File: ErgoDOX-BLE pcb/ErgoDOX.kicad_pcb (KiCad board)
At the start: 2 copper layers, 182.8 x 158.9 mm, 110 parts, among them J1 Conn_01x04, J2 Conn_01x02_Female, J3 Conn_01x02_Female, J4 Conn_01x02, J5 Conn_01x02, P1 USB_C_Plug_USB2.0, Q1 Q_NPN_BCE, SW0:10 SW0:3, SW0:11 SW0:2, SW0:12 SW0:1, SW0:7 SW0:6, SW0:8 SW0:5, SW0:9 SW0:4, SW1:10 SW1:3, SW1:11 SW1:2, SW1:12 SW1:1, SW1:13 SW1:0, SW1:9 SW1:4, SW2:10 SW2:3, SW2:11 SW2:2, SW2:12 SW2:1, SW2:13 SW2:0, SW2:7 SW2:6, SW2:8 SW2:5, SW2:9 SW2:4, SW3:10 SW3:3, SW3:11 SW3:2, SW3:12 SW3:1, SW3:13 SW3:0, SW3:8 SW3:5, SW3:9 SW3:4, SW4:10 SW4:3, SW4:11 SW4:2, SW4:12 SW4:1, SW4:13 SW4:0, SW4:7 SW4:6, SW4:8 SW4:5, SW4:9 SW4:4, SW5:10 SW5:3, SW5:11 SW5:2, SW5:12 SW5:1, SW5:13 SW5:0, SW5:7 SW5:6, SW5:8 SW5:5, SW5:9 SW5:4, U1 MCP23018, U3 C0720B001F

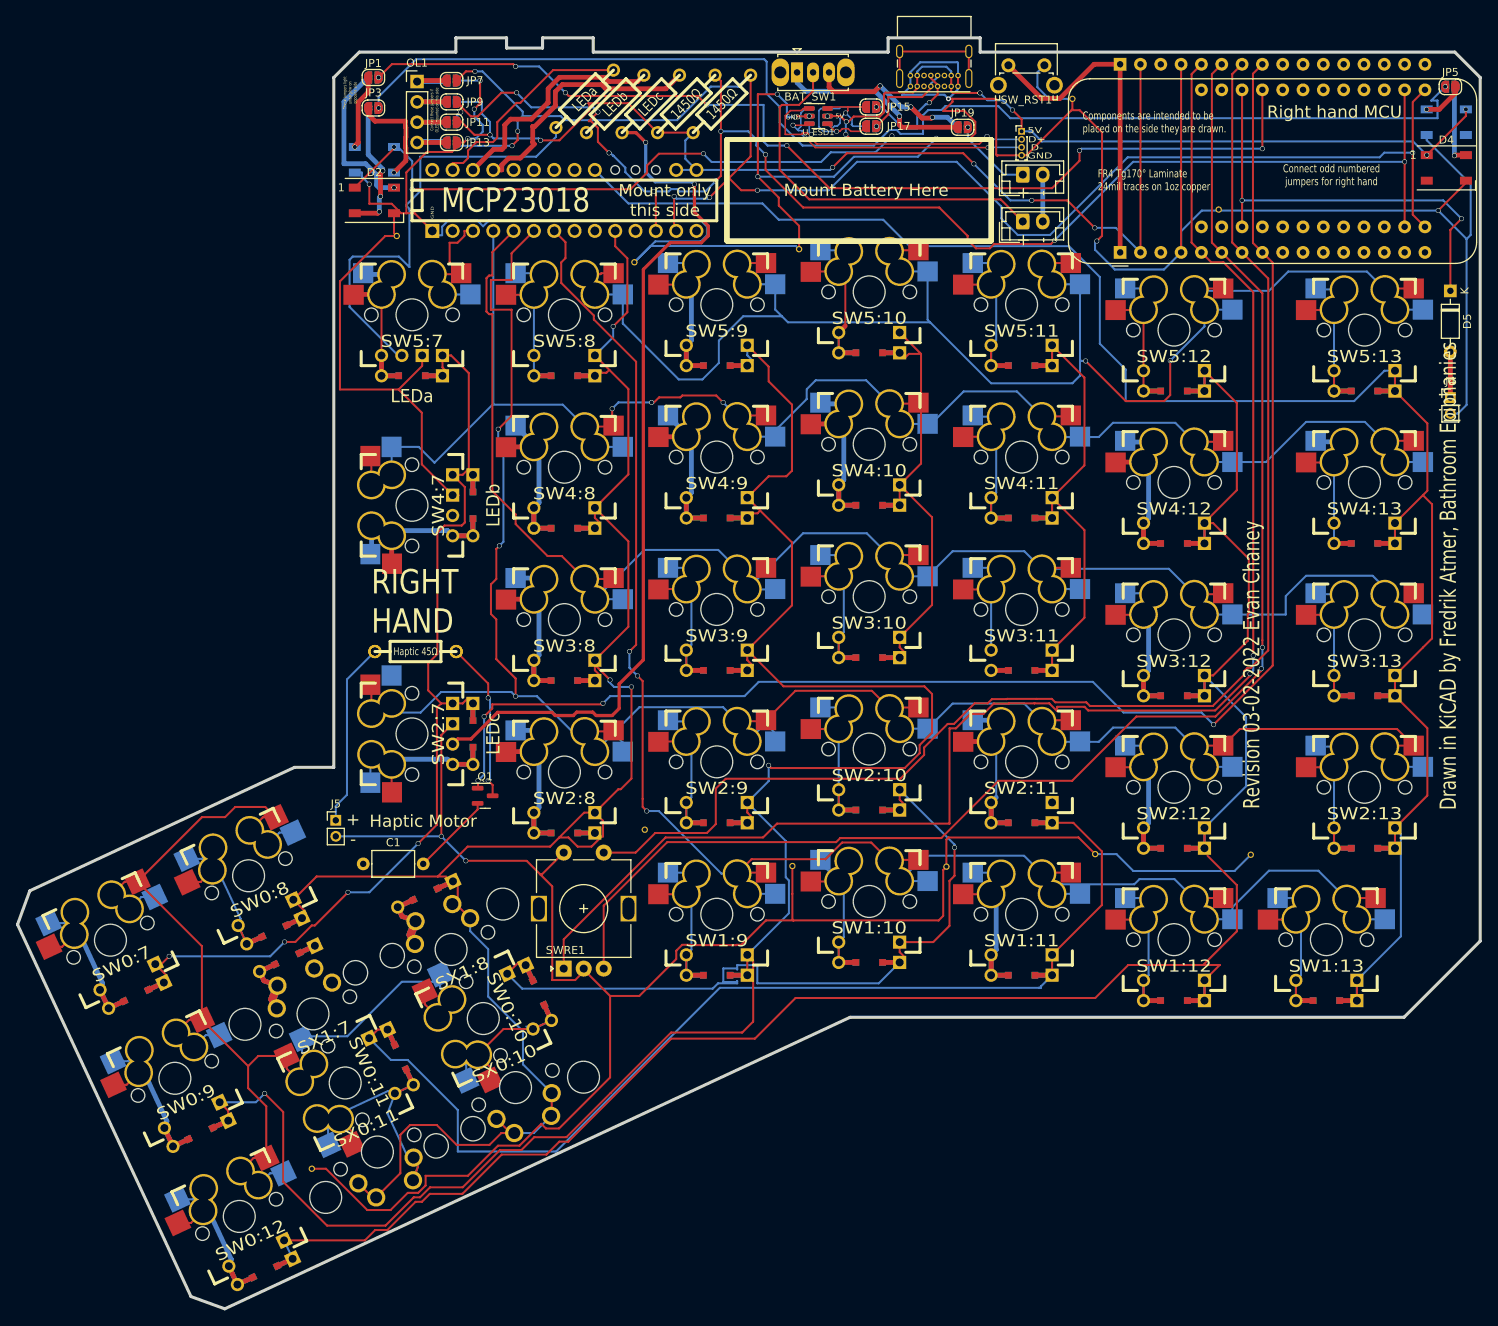
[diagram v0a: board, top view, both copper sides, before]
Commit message: Route me daddy
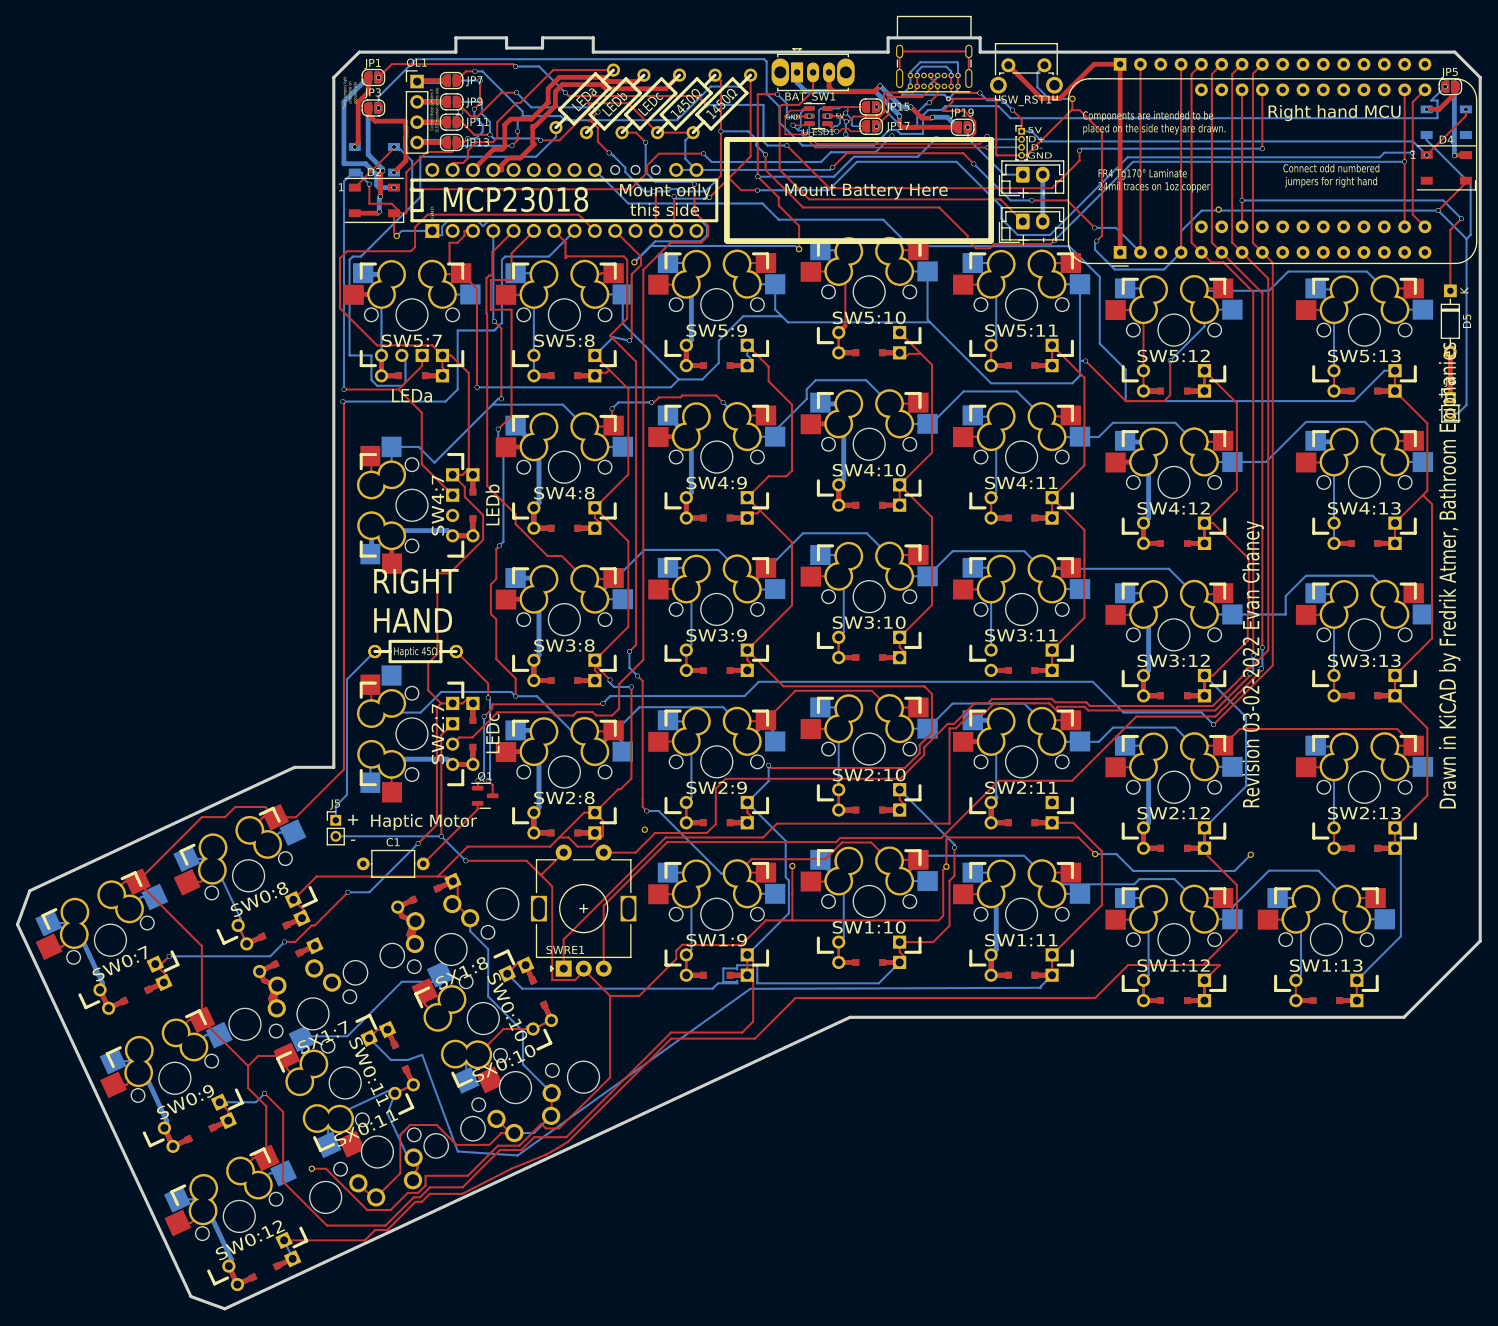
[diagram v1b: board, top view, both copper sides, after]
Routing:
- net /ROW0: track 139.8 -> 243.9 mm, vias 0 -> 1
- net /COL6: track 116.4 -> 175.9 mm
- net /COL3: track 92.1 -> 143.1 mm
- net /ROW4: track 255.8 -> 206.9 mm, vias 3 -> 5
- net /ROW5: track 222.4 -> 263.1 mm, vias 2 -> 3
- net /ROW1: track 218.1 -> 224.0 mm
- net Net-(LED_A1-Pad1): track 57.0 -> 62.4 mm
- net GND: track 661.7 -> 666.6 mm, vias 14 -> 15
- net /COL5: track 218.9 -> 222.0 mm
- net /COL1: track 250.7 -> 249.6 mm
- net /COL2: track 179.1 -> 178.0 mm

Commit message: Everything is connected
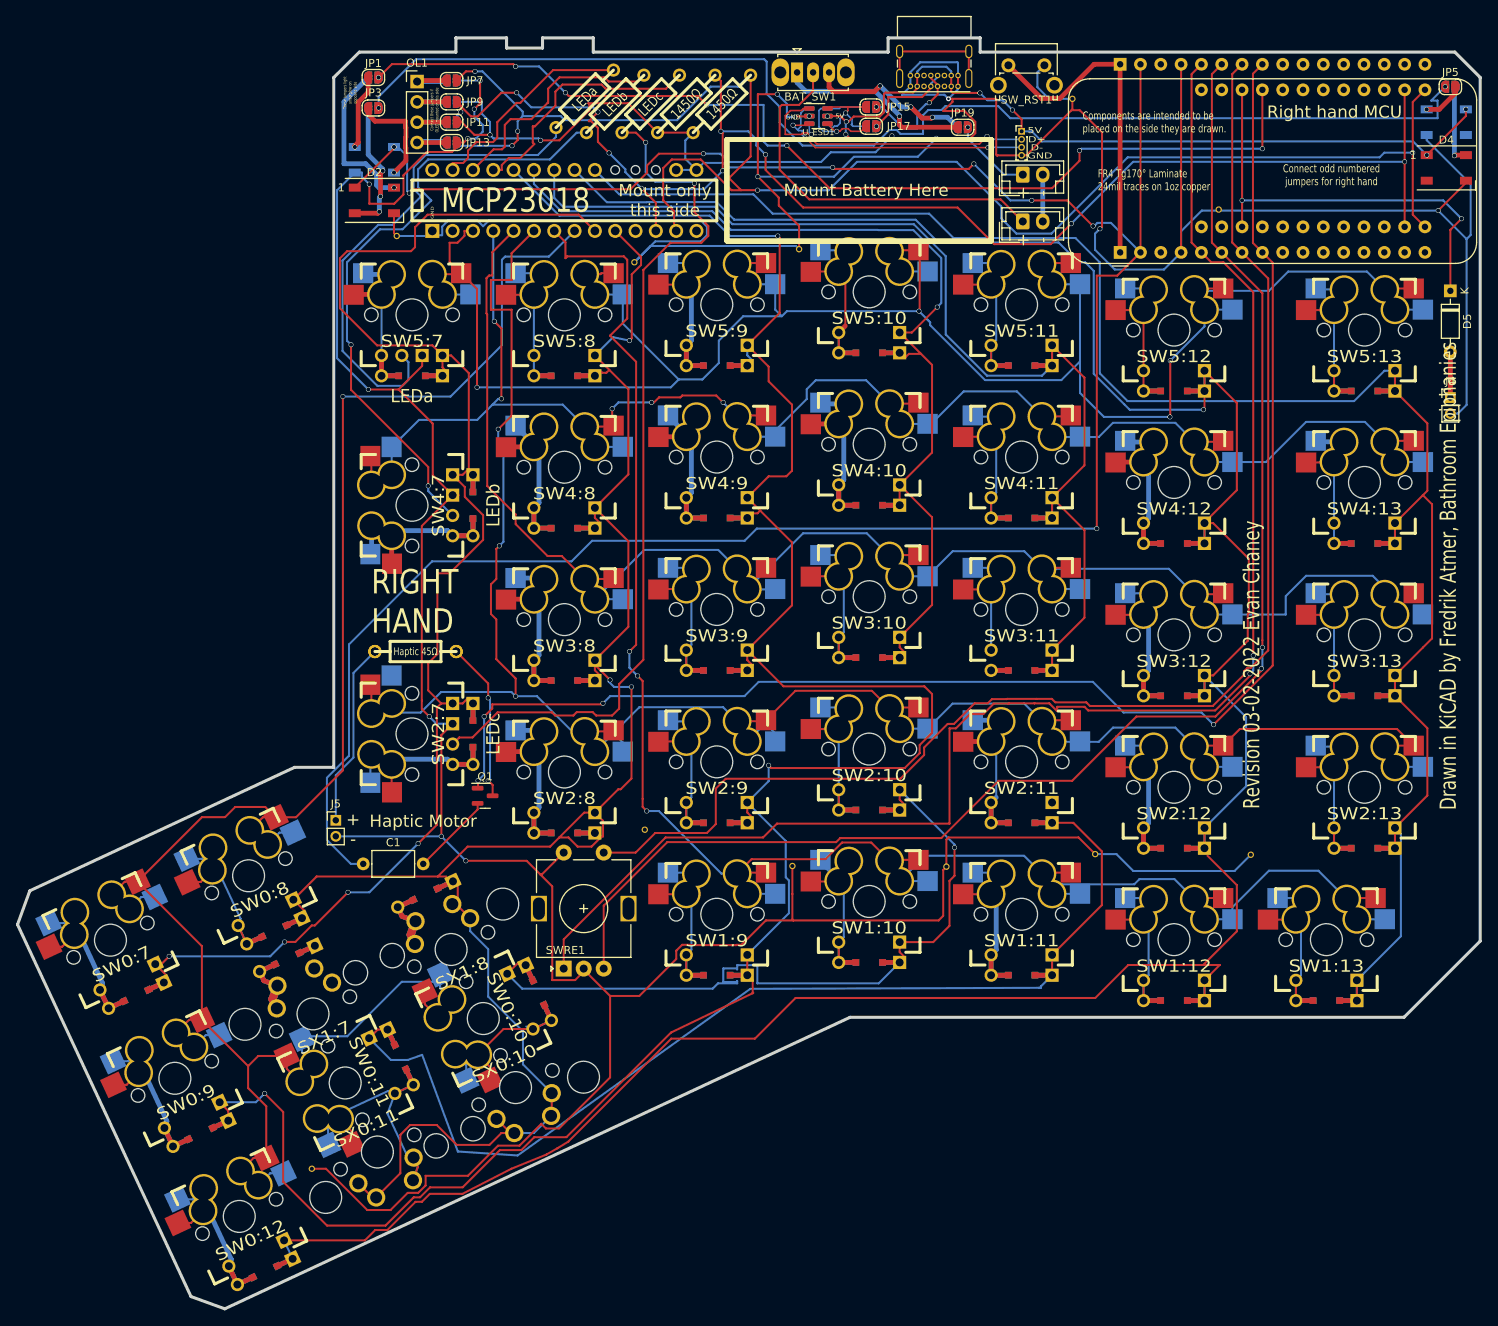
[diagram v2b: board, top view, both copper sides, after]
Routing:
- net +3V3: track 135.0 -> 304.2 mm, vias 6 -> 7
- net /COL1: track 249.6 -> 349.8 mm, vias 0 -> 1
- net /COL2: track 178.0 -> 258.2 mm
- net Net-(LED_B1-Pad1): track 0.00 -> 78.4 mm, vias 0 -> 2
- net /COL3: track 143.1 -> 212.0 mm, vias 1 -> 2
- net /COL4: track 240.6 -> 287.3 mm, vias 2 -> 3
- net GND: track 666.6 -> 695.8 mm, vias 15 -> 16
- net /SDA: track 194.5 -> 202.3 mm, vias 7 -> 5
- net /ROW5: track 263.1 -> 269.6 mm, vias 3 -> 4
- net /ROW0: track 243.9 -> 241.2 mm
- net /ROW4: track 206.9 -> 205.3 mm
- net /COL0: track 231.0 -> 231.9 mm
- net +5V: track 180.2 -> 181.1 mm
